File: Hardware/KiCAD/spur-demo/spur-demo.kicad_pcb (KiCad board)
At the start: 2 copper layers, 63.8 x 105.5 mm, 75 parts, among them IC1 BQ24193RGER, IC2 PCF8575PWR, IC3 ISL91127IRNZ-T7A, J1 SSD1306 Module, J12 USB_C_Plug_USB2.0, J2 Conn_Coaxial, J4 VMA309 Module, J5 Conn_01x02, J6 Conn_01x08_Socket, J7 PAM8392A Module, J8 1x15, J9 1x15, Q1 ZXMN2A01F, SW23 RotaryEncoder_Switch, U1 SA868, U4 LM393, U5 XCVR_ESP32-C3-DEVKITM-1

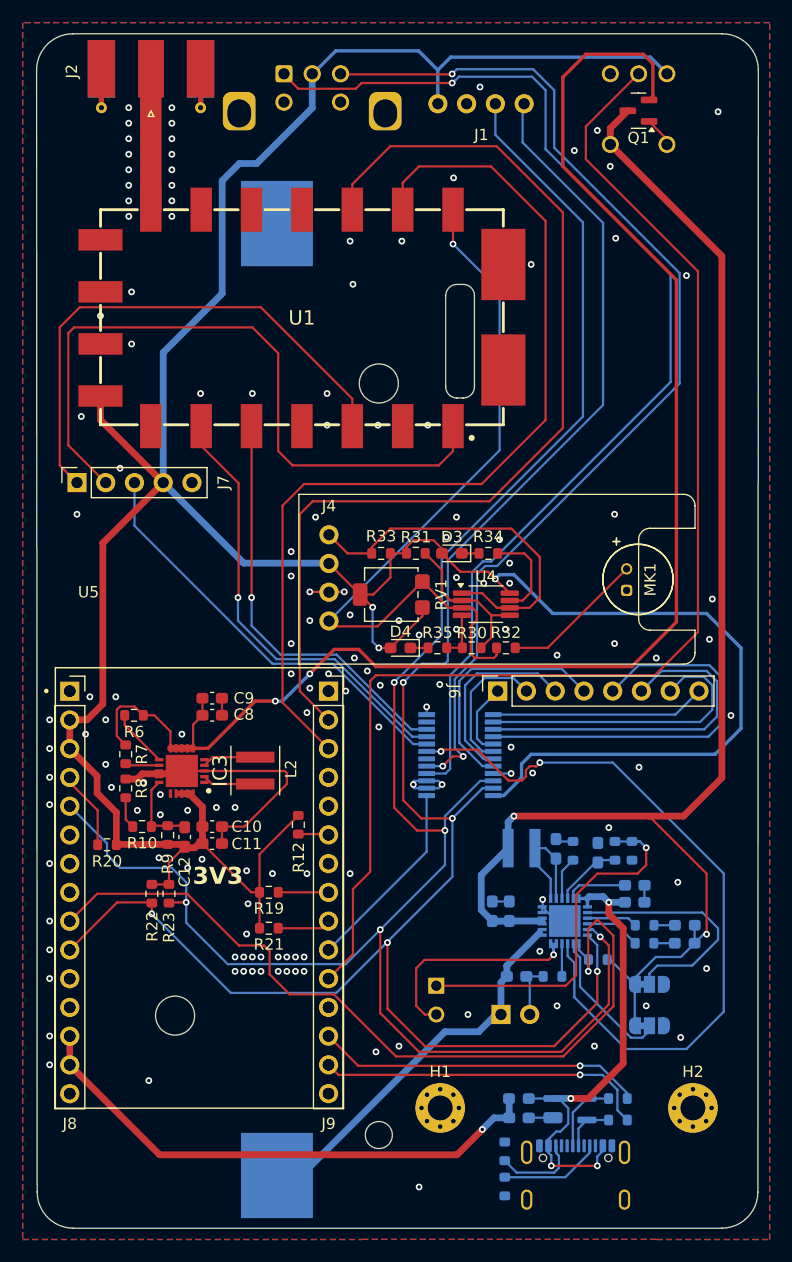
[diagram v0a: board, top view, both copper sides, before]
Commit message: fix: disconnect unused COL5 of switch matrix in favor of encoder switch
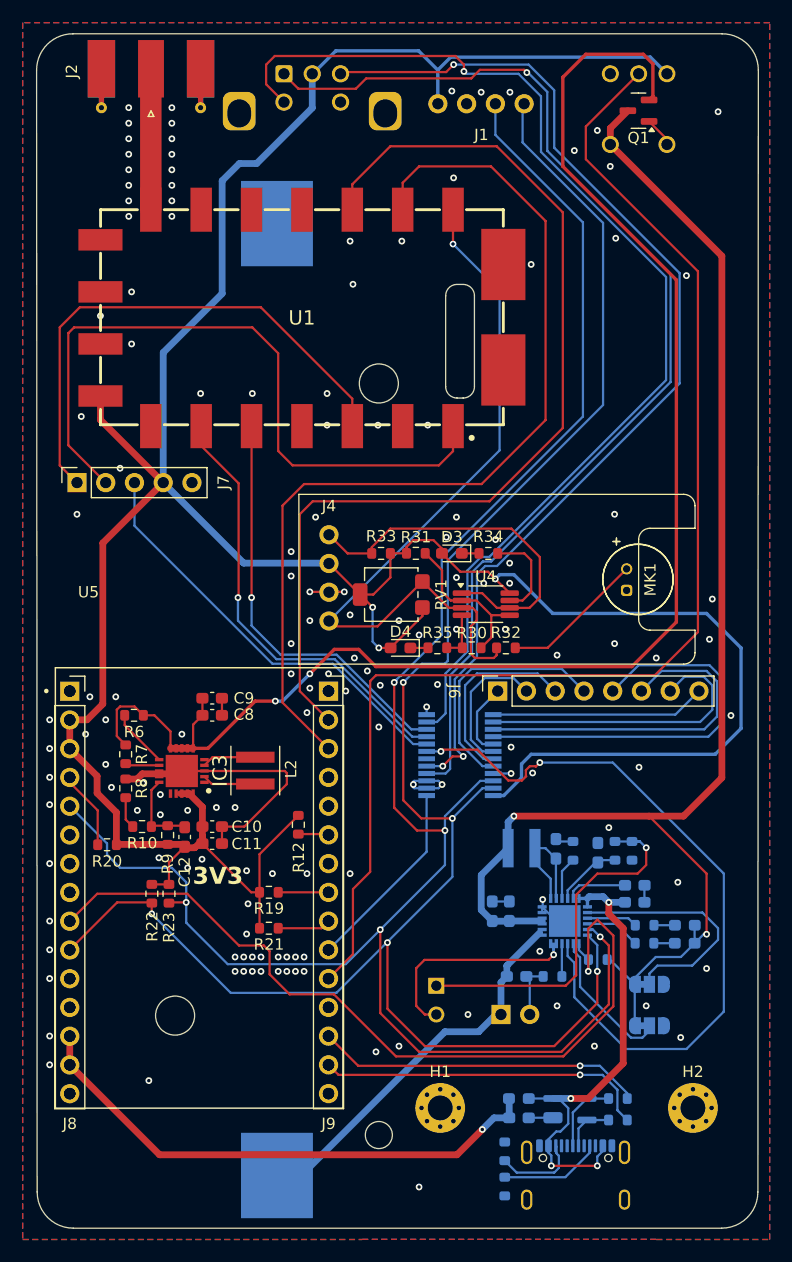
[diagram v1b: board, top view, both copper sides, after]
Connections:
- IC2 pad 11: /Keypad/COL5 -> /ENC_SW
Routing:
- net /ENC_SW: track 0.00 -> 100.0 mm, vias 0 -> 1
- net /ENC_CLK: track 99.9 -> 100.4 mm
- net GND: vias 146 -> 148
